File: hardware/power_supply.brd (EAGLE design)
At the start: 76.2 x 38.1 mm, 38 parts, among them Q1 IRF630N, SW1 T411001B, SW2 T411001B, U1 MC34063, U2 AP1507, U3 CD40109B_SPLITEN

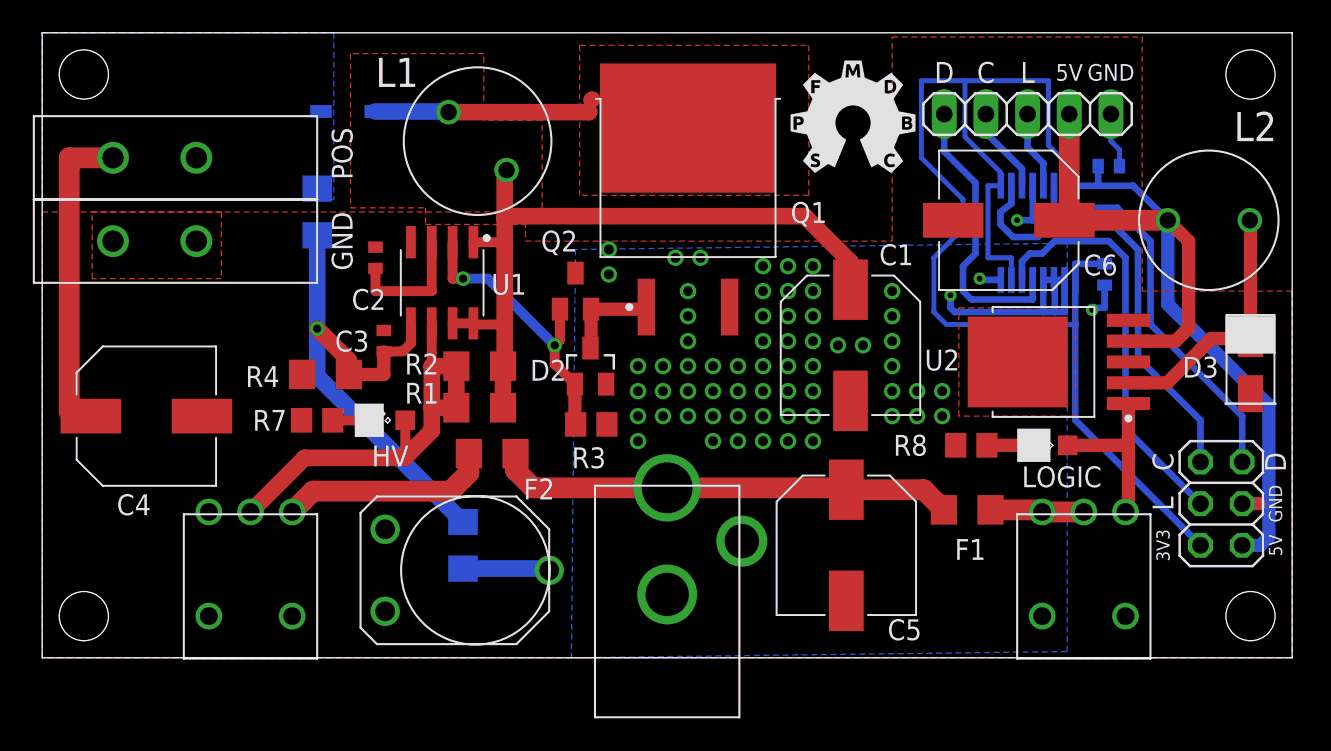
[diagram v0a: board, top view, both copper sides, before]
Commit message: Final update before submitting to PCB shop
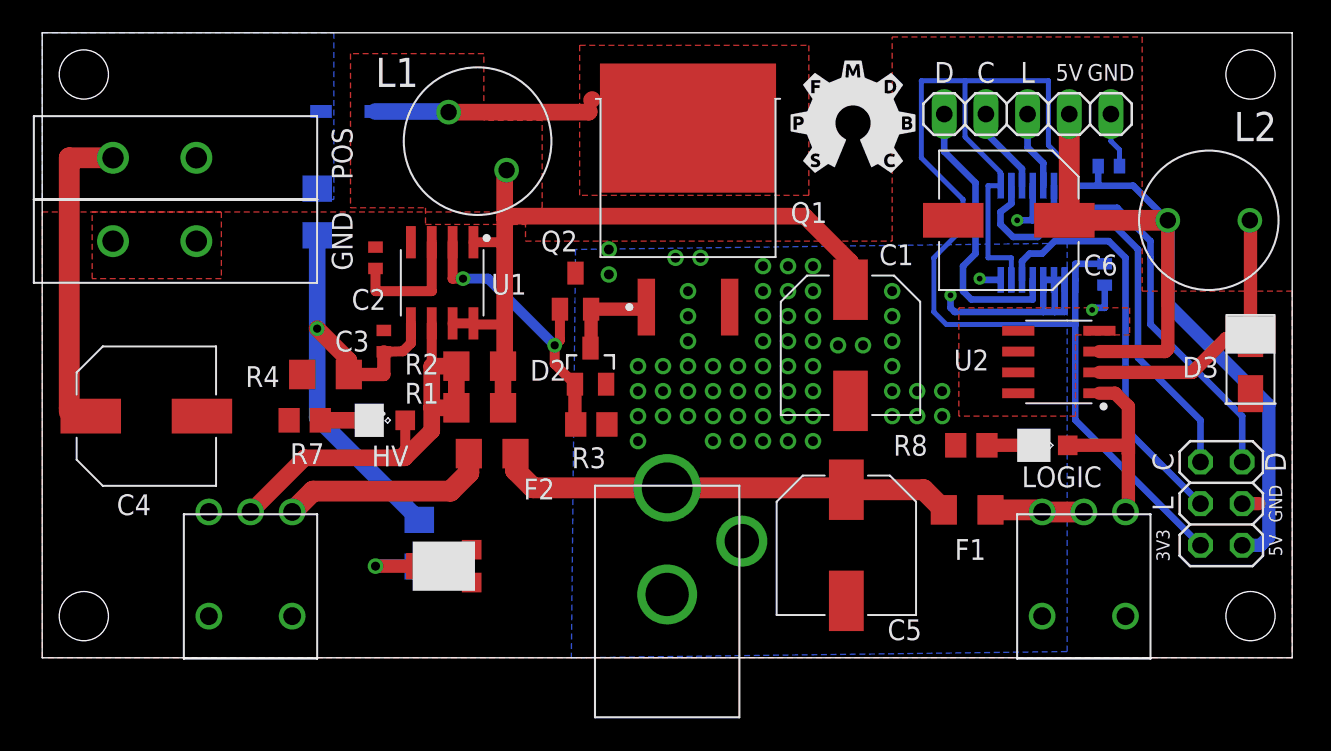
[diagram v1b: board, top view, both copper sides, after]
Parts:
- RX: device nixie_ticker:3309P-1-202 -> nixie_ticker:TC33X-2
- U2: value AP1507 -> AP1507SOIC-8; device nixie_ticker:TO127P990X239-6 -> nixie_ticker:SOIC127P600X175-8
- moved R6 2.67 mm to (23.0, 6.99)
- moved RX 1.55 mm to (24.4, 5.59), turned to 90 degrees
- moved R7 0.76 mm to (16.0, 14.5)
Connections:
- net +5V: now also U2.3; no longer U2.4
- net GND: now also U2.4, U2.7, U2.8; no longer U2.3
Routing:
- net N$8: track 10.4 -> 12.8 mm
- net N$10: track 15.8 -> 17.3 mm
- net GND: track 27.5 -> 26.0 mm
- net N$9: track 31.3 -> 30.1 mm
- net +5V: track 55.5 -> 56.5 mm
- net N$11: track 2.32 -> 3.08 mm
- net N$3: track 5.30 -> 5.29 mm, vias 0 -> 1

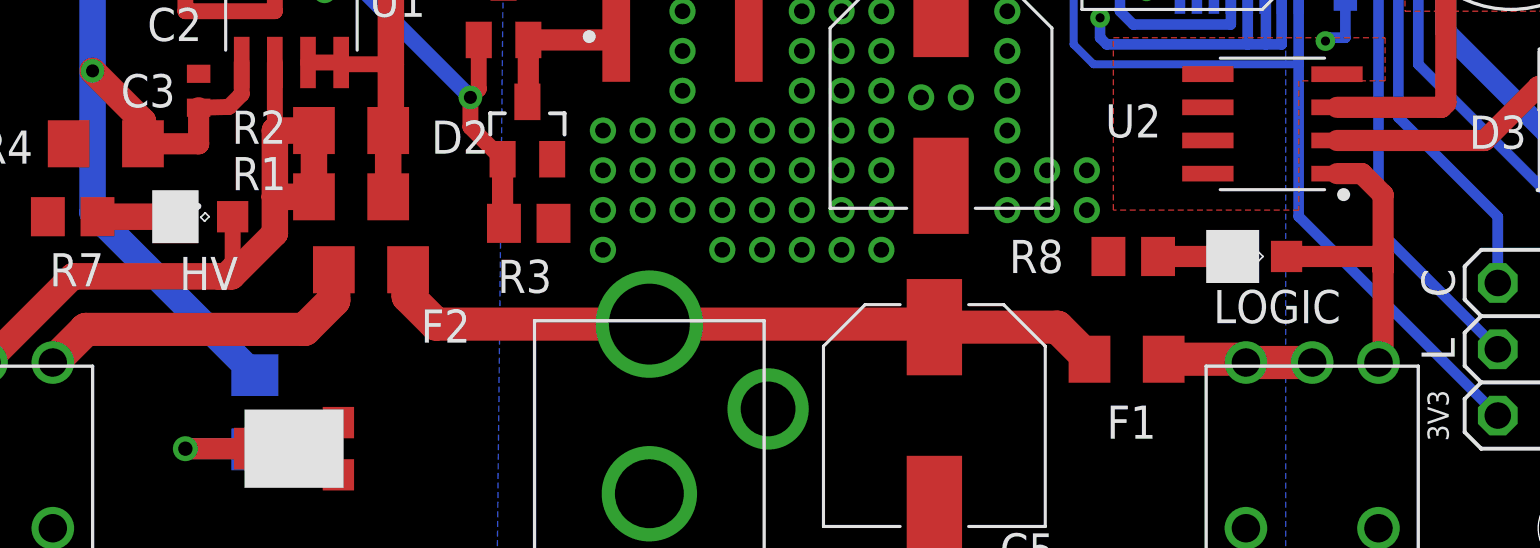
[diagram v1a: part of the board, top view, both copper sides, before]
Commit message: Updates 8-28
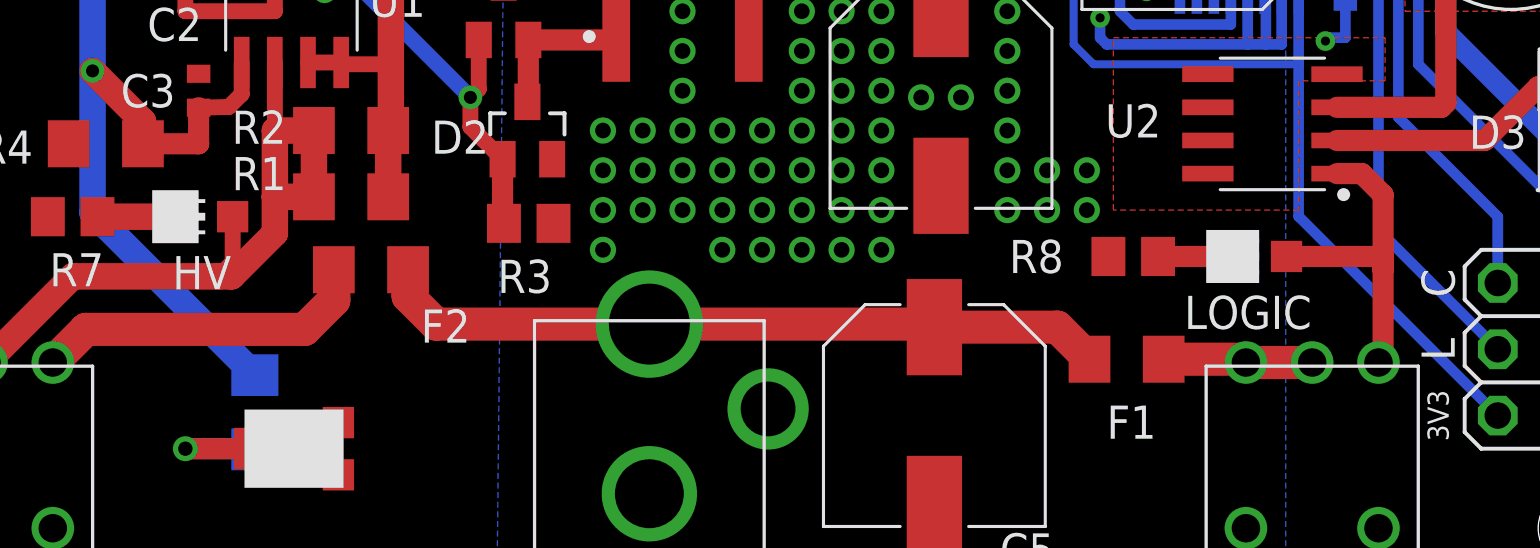
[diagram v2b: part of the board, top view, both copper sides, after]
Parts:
- C2, C3: device resistor:C0402 -> nixie_ticker:C0402
- C7, C8: value (none) -> 1uF; device resistor:C0402 -> nixie_ticker:C0402
- HV, LOGIC: device led:SML0805 -> led:CHIP-LED0805
- turned HV to 90 degrees
- turned LOGIC to 90 degrees
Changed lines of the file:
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@@
 </layers>
 <board>
-<fusionsync huburn="a.cGVyc29uYWw6dWUyYTY5OTEw" projecturn="a.cGVyc29uYWw6dWUyYTY5OTEwIzIwMTgwNjMwMTM4MzExNzgx" f3durn="urn:adsk.wipprod:dm.lineage:bjyJQ3K9ReGs7_9rgABCYQ" pcbguid="75b782bf-6294-4662-834a-dbb7a3b1e7c4" lastpulledtime="" lastsyncedchangeguid="4c63b08d-e52d-0b9f-0fa0-2ec24846586d"/>
+<fusionsync huburn="a.cGVyc29uYWw6dWUyYTY5OTEw" projecturn="a.cGVyc29uYWw6dWUyYTY5OTEwIzIwMTgwNjMwMTM4MzExNzgx" f3durn="urn:adsk.wipprod:dm.lineage:bjyJQ3K9ReGs7_9rgABCYQ" pcbguid="75b782bf-6294-4662-834a-dbb7a3b1e7c4" lastpulledtime="" lastsyncedchangeguid="97ed7a0b-55a9-dae0-7aa2-698207faa45f"/>
 <plain>
 <wire x1="0" y1="0" x2="76.2" y2="0" width="0" layer="20"/>
@@
 <text x="38.1" y="36.172225" size="1.6764" layer="22" font="vector" rot="MR0" align="center">https://github.com/bmboucher/nixie_ticker</text>
 <rectangle x1="19.05" y1="13.462" x2="20.828" y2="15.494" layer="21"/>
-<rectangle x1="59.436" y1="11.938" x2="61.468" y2="13.97" layer="21"/>
+<rectangle x1="59.436" y1="11.938" x2="61.468" y2="13.97" layer="21" rot="R90"/>
 <circle x="62.23" y="24.892" radius="0.762" width="0.4064" layer="22"/>
 <rectangle x1="47.099221875" y1="29.55798125" x2="47.129703125" y2="29.57321875" layer="21"/>
@@
 <attribute name="NAME" x="52.07" y="23.935" size="1.27" layer="25" font="vector" align="bottom-center"/>
 </element>
-<element name="C2" library="resistor" library_urn="urn:adsk.eagle:library:348" package="C0402" package3d_urn="urn:adsk.eagle:package:23626/1" value="680pF" x="20.32" y="24.384" smashed="yes" rot="R90">
+<element name="C2" library="nixie_ticker" library_urn="urn:adsk.eagle:library:3857935" package="C0402" package3d_urn="urn:adsk.eagle:package:4771247/2" value="680pF" x="20.32" y="24.384" smashed="yes" rot="R90">
 <attribute name="NAME" x="20.955" y="22.479" size="1.27" layer="25" font="vector" rot="R180"/>
 <attribute name="VALUE" x="22.225" y="23.749" size="1.27" layer="27" rot="R90"/>
 </element>
-<element name="C3" library="resistor" library_urn="urn:adsk.eagle:library:348" package="C0402" package3d_urn="urn:adsk.eagle:package:23626/1" value="0.01uF" x="20.828" y="19.304" smashed="yes" rot="R90">
+<element name="C3" library="nixie_ticker" library_urn="urn:adsk.eagle:library:3857935" package="C0402" package3d_urn="urn:adsk.eagle:package:4771247/2" value="0.01uF" x="20.828" y="19.304" smashed="yes" rot="R90">
 <attribute name="NAME" x="19.939" y="19.939" size="1.27" layer="25" font="vector" rot="R180"/>
 <attribute name="VALUE" x="22.733" y="18.669" size="1.27" layer="27" rot="R90"/>
@@
 <attribute name="VALUE" x="67.437" y="13.208" size="1.27" layer="27" rot="R270"/>
 </element>
-<element name="HV" library="led" library_urn="urn:adsk.eagle:library:259" package="SML0805" package3d_urn="urn:adsk.eagle:package:15830/1" value="" x="21.082" y="14.478" smashed="yes">
-<attribute name="NAME" x="20.09" y="11.668" size="1.27" layer="25" font="vector"/>
-<attribute name="VALUE" x="19.582" y="12.478" size="1.27" layer="27"/>
-</element>
-<element name="LOGIC" library="led" library_urn="urn:adsk.eagle:library:259" package="SML0805" package3d_urn="urn:adsk.eagle:package:15830/1" value="" x="61.468" y="12.954" smashed="yes">
-<attribute name="NAME" x="59.714" y="10.398" size="1.27" layer="25" font="vector"/>
-<attribute name="VALUE" x="59.968" y="10.954" size="1.27" layer="27"/>
+<element name="HV" library="led" library_urn="urn:adsk.eagle:library:259" package="CHIP-LED0805" package3d_urn="urn:adsk.eagle:package:15818/2" value="" x="21.082" y="14.478" smashed="yes" rot="R90">
+<attribute name="NAME" x="22.074" y="12.97" size="1.27" layer="25" font="vector" rot="R180"/>
+<attribute name="VALUE" x="23.082" y="12.978" size="1.27" layer="27" rot="R90"/>
+</element>
+<element name="LOGIC" library="led" library_urn="urn:adsk.eagle:library:259" package="CHIP-LED0805" package3d_urn="urn:adsk.eagle:package:15818/2" value="" x="61.468" y="12.954" smashed="yes" rot="R90">
+<attribute name="NAME" x="63.476" y="11.446" size="1.27" layer="25" font="vector" rot="R180"/>
+<attribute name="VALUE" x="63.468" y="11.454" size="1.27" layer="27" rot="R90"/>
 </element>
 <element name="R7" library="resistor" library_urn="urn:adsk.eagle:library:348" package="R0805" package3d_urn="urn:adsk.eagle:package:23553/2" value="2k" x="16.002" y="14.478" smashed="yes">
@@
 <attribute name="VALUE" x="66.421" y="36.322" size="1.27" layer="27" rot="R180"/>
 </element>
-<element name="C7" library="resistor" library_urn="urn:adsk.eagle:library:348" package="C0402" package3d_urn="urn:adsk.eagle:package:23626/1" value="" x="64.77" y="23.368" smashed="yes" rot="MR270">
+<element name="C7" library="nixie_ticker" library_urn="urn:adsk.eagle:library:3857935" package="C0402" package3d_urn="urn:adsk.eagle:package:4771247/2" value="1uF" x="64.77" y="23.368" smashed="yes" rot="MR270">
 <attribute name="NAME" x="65.913" y="24.003" size="1.27" layer="26" font="vector" rot="MR180"/>
 <attribute name="VALUE" x="66.675" y="24.003" size="1.27" layer="28" rot="MR270"/>
 </element>
-<element name="C8" library="resistor" library_urn="urn:adsk.eagle:library:348" package="C0402" package3d_urn="urn:adsk.eagle:package:23626/1" value="" x="65.024" y="29.972" smashed="yes" rot="MR180">
+<element name="C8" library="nixie_ticker" library_urn="urn:adsk.eagle:library:3857935" package="C0402" package3d_urn="urn:adsk.eagle:package:4771247/2" value="1uF" x="65.024" y="29.972" smashed="yes" rot="MR180">
 <attribute name="NAME" x="64.389" y="28.956" size="1.27" layer="26" font="vector" rot="MR180"/>
 <attribute name="VALUE" x="64.389" y="31.877" size="1.27" layer="28" rot="MR180"/>
